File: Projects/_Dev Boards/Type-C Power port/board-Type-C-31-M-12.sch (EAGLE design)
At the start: 2 parts, among them J1 USB-TYPE-C-31-M-12

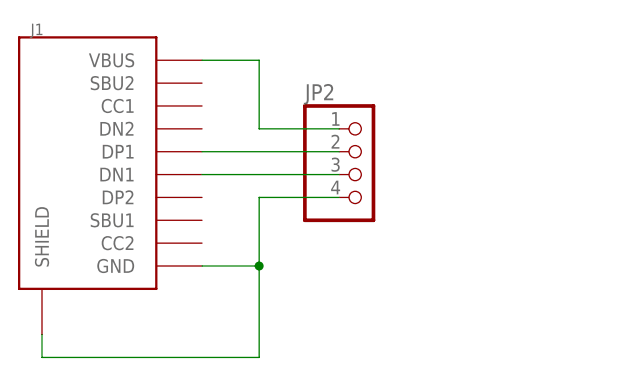
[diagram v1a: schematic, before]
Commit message: update
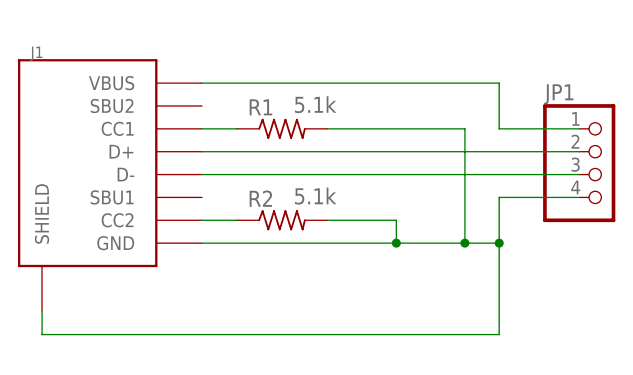
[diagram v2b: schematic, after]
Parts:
- removed JP2: (no value), pinhead_v2:PINHD-1X4/OCT
- added JP1: (no value), angrypig7-Connectors-PinHeads:PINHD-1X4
- added R1, R2: 5.1k, angrypig7-RCL:RR0603
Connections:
- removed net N$1: J1.VBUS, JP2.1
- removed net N$4: J1.GND, J1.SHIELD, JP2.4
- new net GND: J1.GND, J1.SHIELD, JP1.4, R1.2, R2.2
- new net N$5: J1.CC1, R1.1
- new net N$6: J1.CC2, R2.1
- new net VBUS: J1.VBUS, JP1.1
- net N$2: now also J1.D+, JP1.2; no longer J1.DP1, JP2.2
- net N$3: now also J1.D-, JP1.3; no longer J1.DN1, JP2.3
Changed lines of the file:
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@@
 <?xml version="1.0" encoding="utf-8"?>
 <!DOCTYPE eagle SYSTEM "eagle.dtd">
-<eagle version="9.6.1">
+<eagle version="9.6.2">
 <drawing>
 <settings>
@@
 <class number="0" name="default" width="0.254" drill="0">
 </class>
-<class number="1" name="power" width="0.4572" drill="0">
+<class number="1" name="power" width="0.4064" drill="0">
 </class>
 </classes>
 <parts>
-<part name="J1" library="angrypig7-Connectors" deviceset="USB-TYPE-C-31-M-12" device=""/>
-<part name="JP2" library="pinhead_v2" deviceset="PINHD-1X4" device="/OCT"/>
+<part name="J1" library="angrypig7-Connectors" deviceset="USB-TYPE-C-31-M-12" device="" package3d_urn="urn:adsk.eagle:package:24334474/2"/>
+<part name="R1" library="angrypig7-RCL" deviceset="R" device="R0603" package3d_urn="urn:adsk.eagle:package:23555/54" value="5.1k"/>
+<part name="R2" library="angrypig7-RCL" deviceset="R" device="R0603" package3d_urn="urn:adsk.eagle:package:23555/54" value="5.1k"/>
+<part name="JP1" library="angrypig7-Connectors-PinHeads" deviceset="PINHD-1X4" device="" package3d_urn="urn:adsk.eagle:package:22407/2"/>
 </parts>
 <sheets>
@@
 <instances>
 <instance part="J1" gate="G$1" x="7.62" y="25.4" smashed="yes">
-<attribute name="NAME" x="2.54" y="39.624" size="1.27" layer="95"/>
-</instance>
-<instance part="JP2" gate="A" x="39.37" y="24.13" smashed="yes">
-<attribute name="NAME" x="33.02" y="32.385" size="1.778" layer="95"/>
-<attribute name="VALUE" x="33.02" y="16.51" size="1.778" layer="96"/>
+<attribute name="NAME" x="2.54" y="37.084" size="1.27" layer="95"/>
+</instance>
+<instance part="R1" gate="G$1" x="30.48" y="29.21" smashed="yes">
+<attribute name="NAME" x="26.67" y="30.7086" size="1.778" layer="95"/>
+<attribute name="VALUE" x="31.75" y="30.988" size="1.778" layer="96"/>
+</instance>
+<instance part="R2" gate="G$1" x="30.48" y="19.05" smashed="yes">
+<attribute name="NAME" x="26.67" y="20.5486" size="1.778" layer="95"/>
+<attribute name="VALUE" x="31.75" y="20.828" size="1.778" layer="96"/>
+</instance>
+<instance part="JP1" gate="A" x="66.04" y="24.13" smashed="yes">
+<attribute name="NAME" x="59.69" y="32.385" size="1.778" layer="95"/>
+<attribute name="VALUE" x="59.69" y="16.51" size="1.778" layer="96"/>
 </instance>
 </instances>
@@
 </busses>
 <nets>
-<net name="N$1" class="1">
-<segment>
+<net name="VBUS" class="1">
+<segment>
+<wire x1="21.59" y1="34.29" x2="54.61" y2="34.29" width="0.1524" layer="91"/>
+<wire x1="54.61" y1="34.29" x2="54.61" y2="29.21" width="0.1524" layer="91"/>
+<wire x1="54.61" y1="29.21" x2="63.5" y2="29.21" width="0.1524" layer="91"/>
 <pinref part="J1" gate="G$1" pin="VBUS"/>
-<wire x1="21.59" y1="36.83" x2="27.94" y2="36.83" width="0.1524" layer="91"/>
-<wire x1="27.94" y1="36.83" x2="27.94" y2="29.21" width="0.1524" layer="91"/>
-<pinref part="JP2" gate="A" pin="1"/>
-<wire x1="27.94" y1="29.21" x2="36.83" y2="29.21" width="0.1524" layer="91"/>
+<pinref part="JP1" gate="A" pin="1"/>
 </segment>
 </net>
 <net name="N$2" class="0">
 <segment>
-<pinref part="J1" gate="G$1" pin="DP1"/>
-<pinref part="JP2" gate="A" pin="2"/>
-<wire x1="21.59" y1="26.67" x2="36.83" y2="26.67" width="0.1524" layer="91"/>
+<wire x1="21.59" y1="26.67" x2="63.5" y2="26.67" width="0.1524" layer="91"/>
+<pinref part="J1" gate="G$1" pin="D+"/>
+<pinref part="JP1" gate="A" pin="2"/>
 </segment>
 </net>
 <net name="N$3" class="0">
 <segment>
-<pinref part="J1" gate="G$1" pin="DN1"/>
-<pinref part="JP2" gate="A" pin="3"/>
-<wire x1="21.59" y1="24.13" x2="36.83" y2="24.13" width="0.1524" layer="91"/>
-</segment>
-</net>
-<net name="N$4" class="1">
-<segment>
+<wire x1="21.59" y1="24.13" x2="63.5" y2="24.13" width="0.1524" layer="91"/>
+<pinref part="J1" gate="G$1" pin="D-"/>
+<pinref part="JP1" gate="A" pin="3"/>
+</segment>
+</net>
+<net name="GND" class="1">
+<segment>
+<wire x1="54.61" y1="21.59" x2="63.5" y2="21.59" width="0.1524" layer="91"/>
+<wire x1="3.81" y1="8.89" x2="3.81" y2="6.35" width="0.1524" layer="91"/>
+<wire x1="3.81" y1="6.35" x2="54.61" y2="6.35" width="0.1524" layer="91"/>
+<wire x1="54.61" y1="6.35" x2="54.61" y2="16.51" width="0.1524" layer="91"/>
 <pinref part="J1" gate="G$1" pin="GND"/>
-<wire x1="21.59" y1="13.97" x2="27.94" y2="13.97" width="0.1524" layer="91"/>
-<wire x1="27.94" y1="13.97" x2="27.94" y2="21.59" width="0.1524" layer="91"/>
-<pinref part="JP2" gate="A" pin="4"/>
-<wire x1="27.94" y1="21.59" x2="36.83" y2="21.59" width="0.1524" layer="91"/>
+<wire x1="54.61" y1="16.51" x2="54.61" y2="21.59" width="0.1524" layer="91"/>
+<wire x1="21.59" y1="16.51" x2="43.18" y2="16.51" width="0.1524" layer="91"/>
+<junction x="54.61" y="16.51"/>
 <pinref part="J1" gate="G$1" pin="SHIELD"/>
-<wire x1="3.81" y1="6.35" x2="3.81" y2="3.81" width="0.1524" layer="91"/>
-<wire x1="3.81" y1="3.81" x2="27.94" y2="3.81" width="0.1524" layer="91"/>
-<wire x1="27.94" y1="3.81" x2="27.94" y2="13.97" width="0.1524" layer="91"/>
-<junction x="27.94" y="13.97"/>
+<pinref part="R1" gate="G$1" pin="2"/>
+<wire x1="43.18" y1="16.51" x2="50.8" y2="16.51" width="0.1524" layer="91"/>
+<wire x1="50.8" y1="16.51" x2="54.61" y2="16.51" width="0.1524" layer="91"/>
+<wire x1="35.56" y1="29.21" x2="50.8" y2="29.21" width="0.1524" layer="91"/>
+<wire x1="50.8" y1="29.21" x2="50.8" y2="16.51" width="0.1524" layer="91"/>
+<junction x="50.8" y="16.51"/>
+<pinref part="R2" gate="G$1" pin="2"/>
+<wire x1="35.56" y1="19.05" x2="43.18" y2="19.05" width="0.1524" layer="91"/>
+<wire x1="43.18" y1="19.05" x2="43.18" y2="16.51" width="0.1524" layer="91"/>
+<junction x="43.18" y="16.51"/>
+<pinref part="JP1" gate="A" pin="4"/>
+</segment>
+</net>
+<net name="N$5" class="0">
+<segment>
+<pinref part="R1" gate="G$1" pin="1"/>
+<pinref part="J1" gate="G$1" pin="CC1"/>
+<wire x1="25.4" y1="29.21" x2="21.59" y2="29.21" width="0.1524" layer="91"/>
+</segment>
+</net>
+<net name="N$6" class="0">
+<segment>
+<pinref part="R2" gate="G$1" pin="1"/>
+<pinref part="J1" gate="G$1" pin="CC2"/>
+<wire x1="25.4" y1="19.05" x2="21.59" y2="19.05" width="0.1524" layer="91"/>
 </segment>
 </net>
@@
 </schematic>
 </drawing>
+<compatibility>
+<note version="8.3" severity="warning">
+Since Version 8.3, EAGLE supports URNs for individual library
+assets (packages, symbols, and devices). The URNs of those assets
+will not be understood (or retained) with this version.
+</note>
+<note version="8.3" severity="warning">
+Since Version 8.3, EAGLE supports the association of 3D packages
+with devices in libraries, schematics, and board files. Those 3D
+packages will not be understood (or retained) with this version.
+</note>
+<note version="8.4" severity="warning">
+Since Version 8.4, EAGLE supports properties for SPICE simulation.
+Probes in schematics and SPICE mapping objects found in parts and library devices
+will not be understood with this version. Update EAGLE to the latest version
+for full support of SPICE simulation.
+</note>
+</compatibility>
 </eagle>
